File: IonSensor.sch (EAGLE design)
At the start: 20 parts, among them IC1 QUAD_OPAMPD, IC2 QUAD_OPAMPD, IC3 QUAD_OPAMPD, X1 JST-XH-04-PIN-LONG-PAD

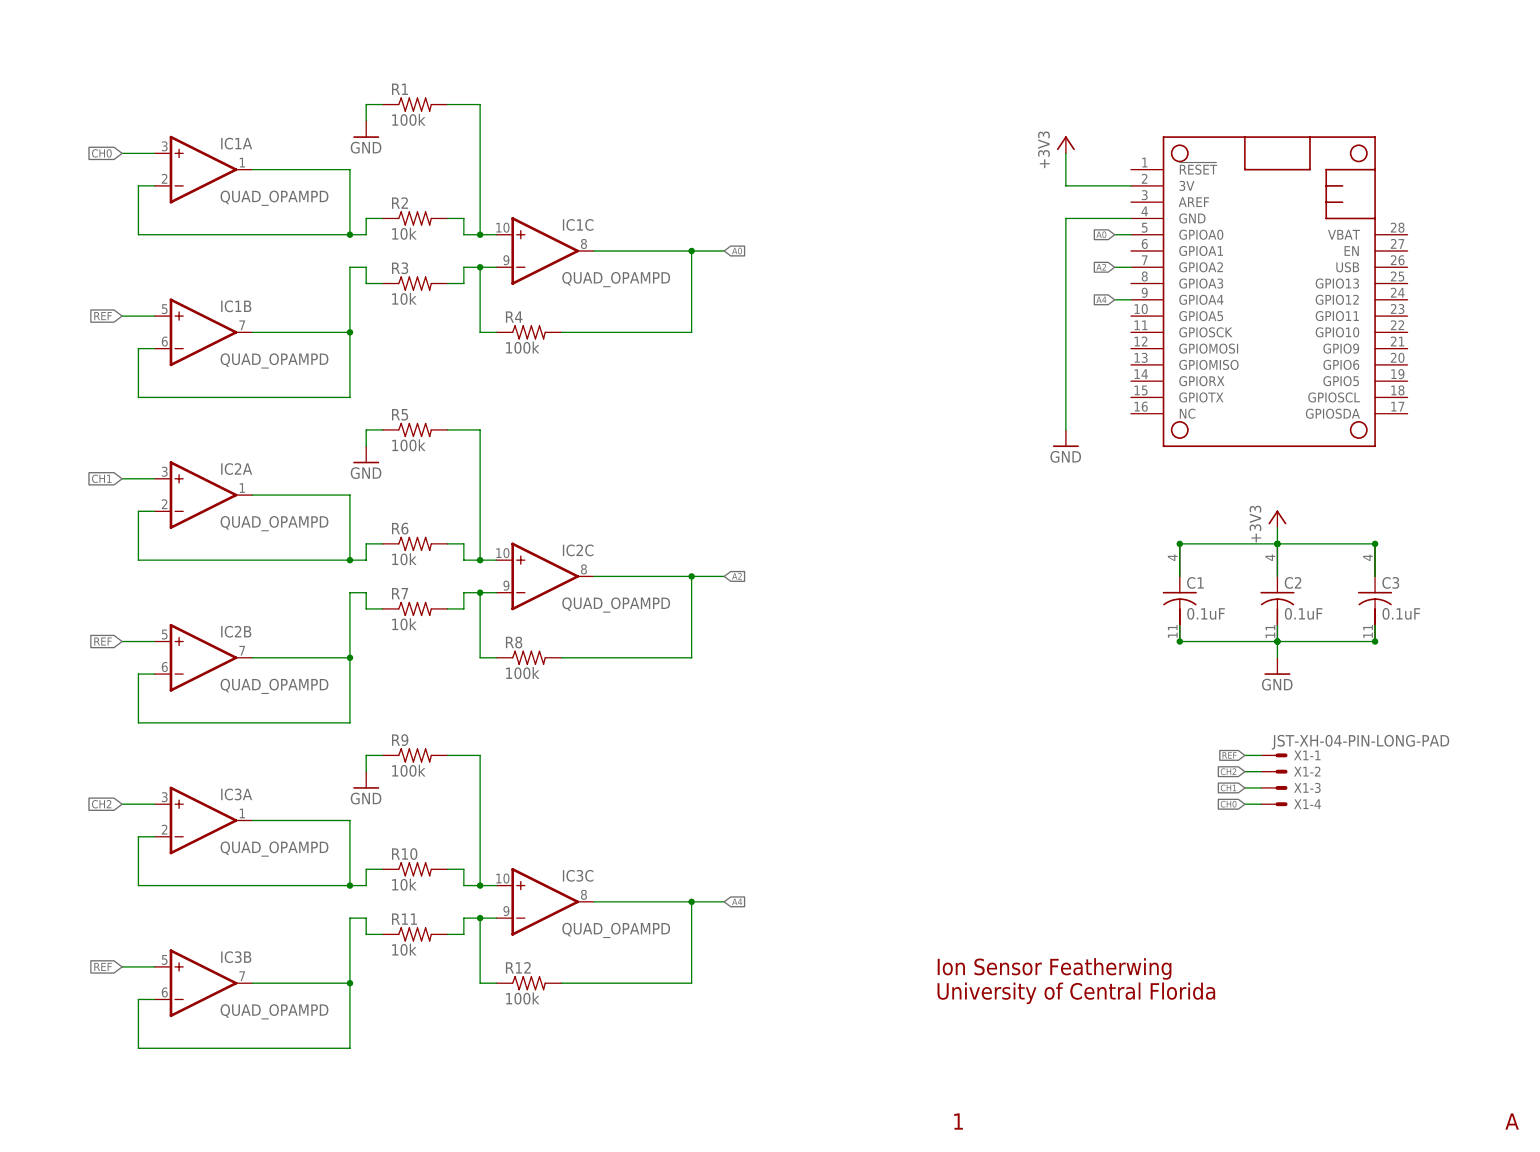
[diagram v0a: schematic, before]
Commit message: Switch to 2 channel opamp
Switched to 2 channel opamp instead of quad opamp.
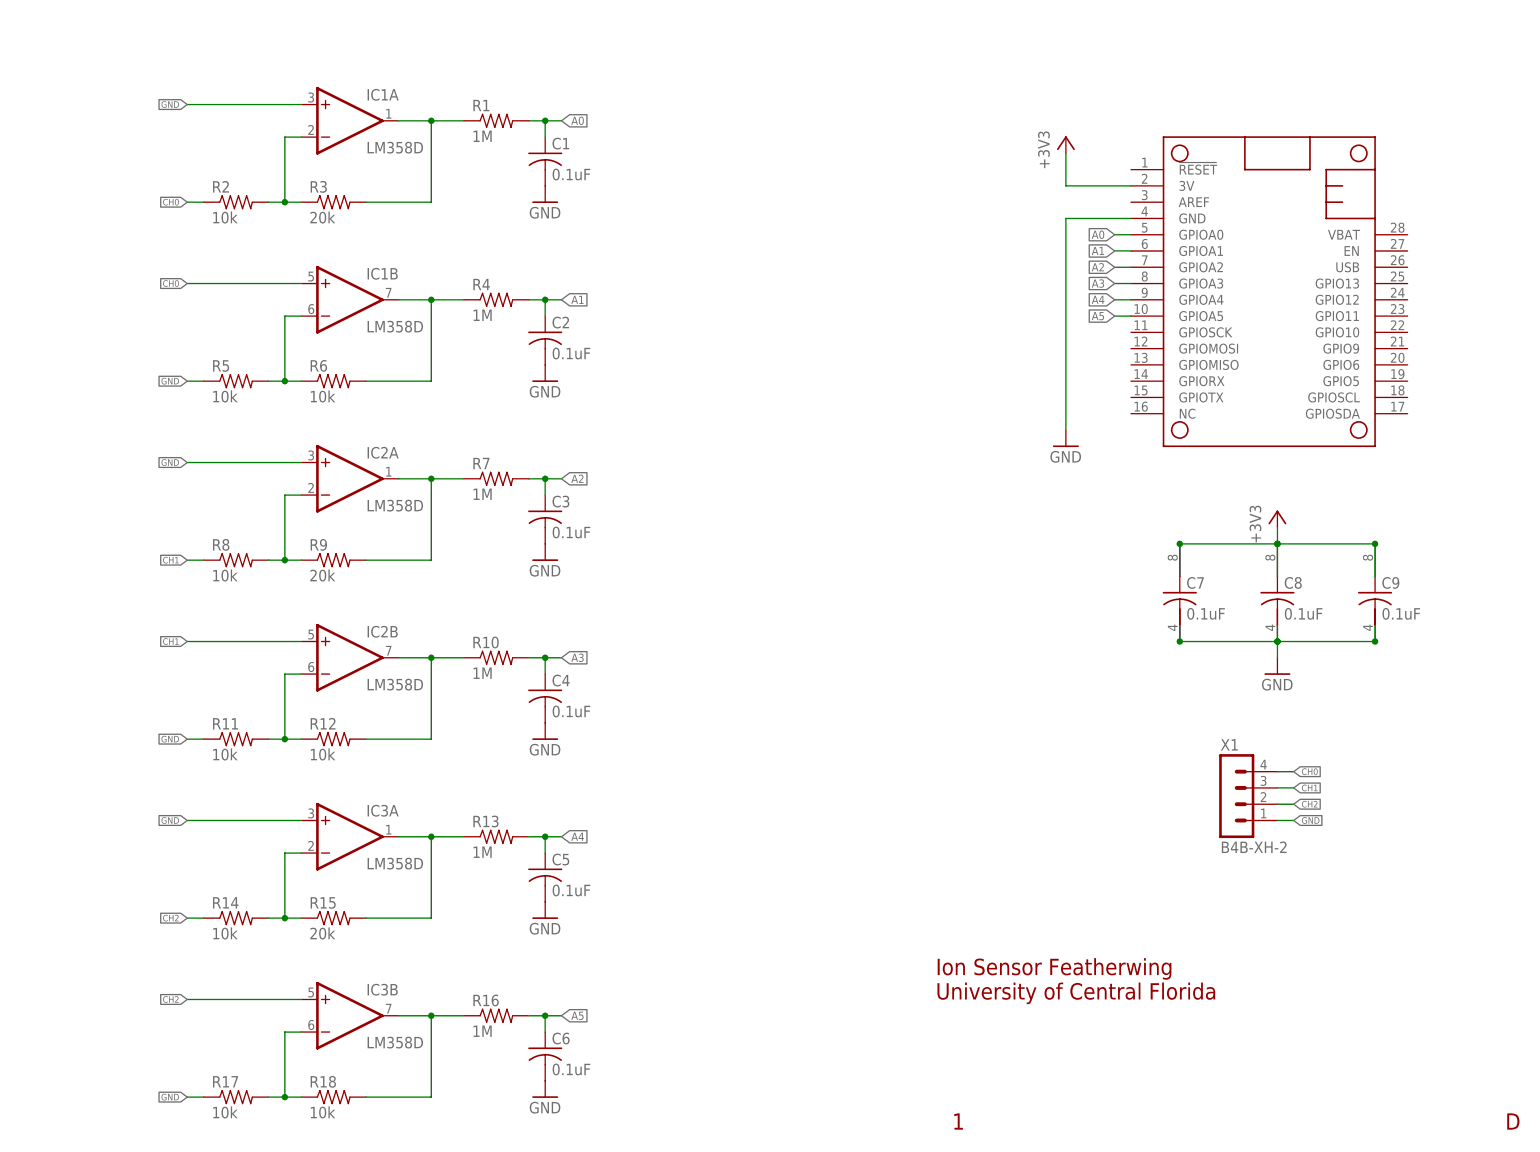
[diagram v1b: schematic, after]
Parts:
- added C4, C5, C6, C7, C8, C9: 0.1uF, adafruit:C-USC0402
- added R13, R16: 1M, adafruit:R-US_R0402
- added R14, R17, R18: 10k, adafruit:R-US_R0402
- added R15: 20k, adafruit:R-US_R0402
- C1, C2, C3: device adafruit:C-USC0603 -> adafruit:C-USC0402
- IC1, IC2, IC3: value QUAD_OPAMPD -> LM358D; device adafruit:QUAD_OPAMPD -> linear:LM358D
- R1, R4: value 100k -> 1M; device adafruit:R-US_R0603 -> adafruit:R-US_R0402
- R10, R7: value 10k -> 1M; device adafruit:R-US_R0603 -> adafruit:R-US_R0402
- R11, R2, R6: device adafruit:R-US_R0603 -> adafruit:R-US_R0402
- R12, R5, R8: value 100k -> 10k; device adafruit:R-US_R0603 -> adafruit:R-US_R0402
- R3: value 10k -> 20k; device adafruit:R-US_R0603 -> adafruit:R-US_R0402
- R9: value 100k -> 20k; device adafruit:R-US_R0603 -> adafruit:R-US_R0402
- X1: value JST-XH-04-PIN-LONG-PAD -> B4B-XH-2; device Rembrandt Electronics - JST XH Connectors v1-0:JST-XH-04-PIN-LONG-PAD -> con-JST XH:B4B-XH-2
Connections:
- removed net N$13: IC3C.+IN, R10.2, R9.2
- removed net N$14: IC3C.-IN, R11.2, R12.1
- removed net REF: IC1B.+IN, IC2B.+IN, IC3B.+IN, X1-1.S
- new net A1: C2.1, MS1.GPIOA1, R4.2
- new net A3: C4.1, MS1.GPIOA3, R10.2
- new net A5: C6.1, MS1.GPIOA5, R16.2
- new net N$10: IC3A.OUT, R13.1, R15.2
- new net N$5: IC2A.-IN, R8.2, R9.1
- net +3V3: now also C7.1, C8.1, C9.1; no longer C1.1, C2.1, C3.1
- net A0: now also C1.1, R1.2; no longer IC1C.OUT, R4.2
- net A2: now also C3.1, R7.2; no longer IC2C.OUT, R8.2
- net A4: now also C5.1, R13.2; no longer IC3C.OUT, R12.2
- net CH0: now also IC1B.+IN, R2.1, X1.4; no longer IC1A.+IN, X1-4.S
- net CH1: now also IC2B.+IN, R8.1, X1.3; no longer IC2A.+IN, X1-3.S
- net CH2: now also IC3B.+IN, R14.1, X1.2; no longer IC3A.+IN, X1-2.S
- net GND: now also C4.2, C5.2, C6.2, C7.2, C8.2, C9.2, IC1A.+IN, IC2A.+IN, IC3A.+IN, R11.1, R17.1, X1.1; no longer R1.1, R9.1
- net N$1: now also R2.2, R3.1; no longer IC1A.OUT, R2.1
- net N$11: now also IC3B.-IN, R17.2, R18.1; no longer IC3A.-IN, IC3A.OUT, R10.1
- net N$12: now also R16.1, R18.2; no longer IC3B.-IN, R11.1
- net N$2: now also IC1B.-IN, R5.2, R6.1; no longer IC1C.+IN, R1.2, R2.2
- net N$3: now also IC1A.OUT, R1.1, R3.2; no longer IC1B.-IN, IC1B.OUT, R3.1
- net N$4: now also IC1B.OUT, R6.2; no longer IC1C.-IN, R3.2
- net N$6: now also R7.1, R9.2; no longer IC2A.-IN, R6.1
- net N$7: now also R11.2, R12.1; no longer IC2B.OUT, R7.1
- net N$8: now also IC2B.OUT, R10.1, R12.2; no longer IC2C.+IN, R5.2, R6.2
- net N$9: now also IC3A.-IN, R14.2, R15.1; no longer IC2C.-IN, R7.2, R8.1
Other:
- note added: "D"
- note removed: "A"
- moved on the sheet: C1, C2, C3, IC1A, IC1B, IC2A, IC2B, IC3A, IC3B, R1, R10, R11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

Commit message: Revert "Switch to 2 channel opamp"
This reverts commit d2c6276b5e9005aaa4bb267ec01d57cf95291150.
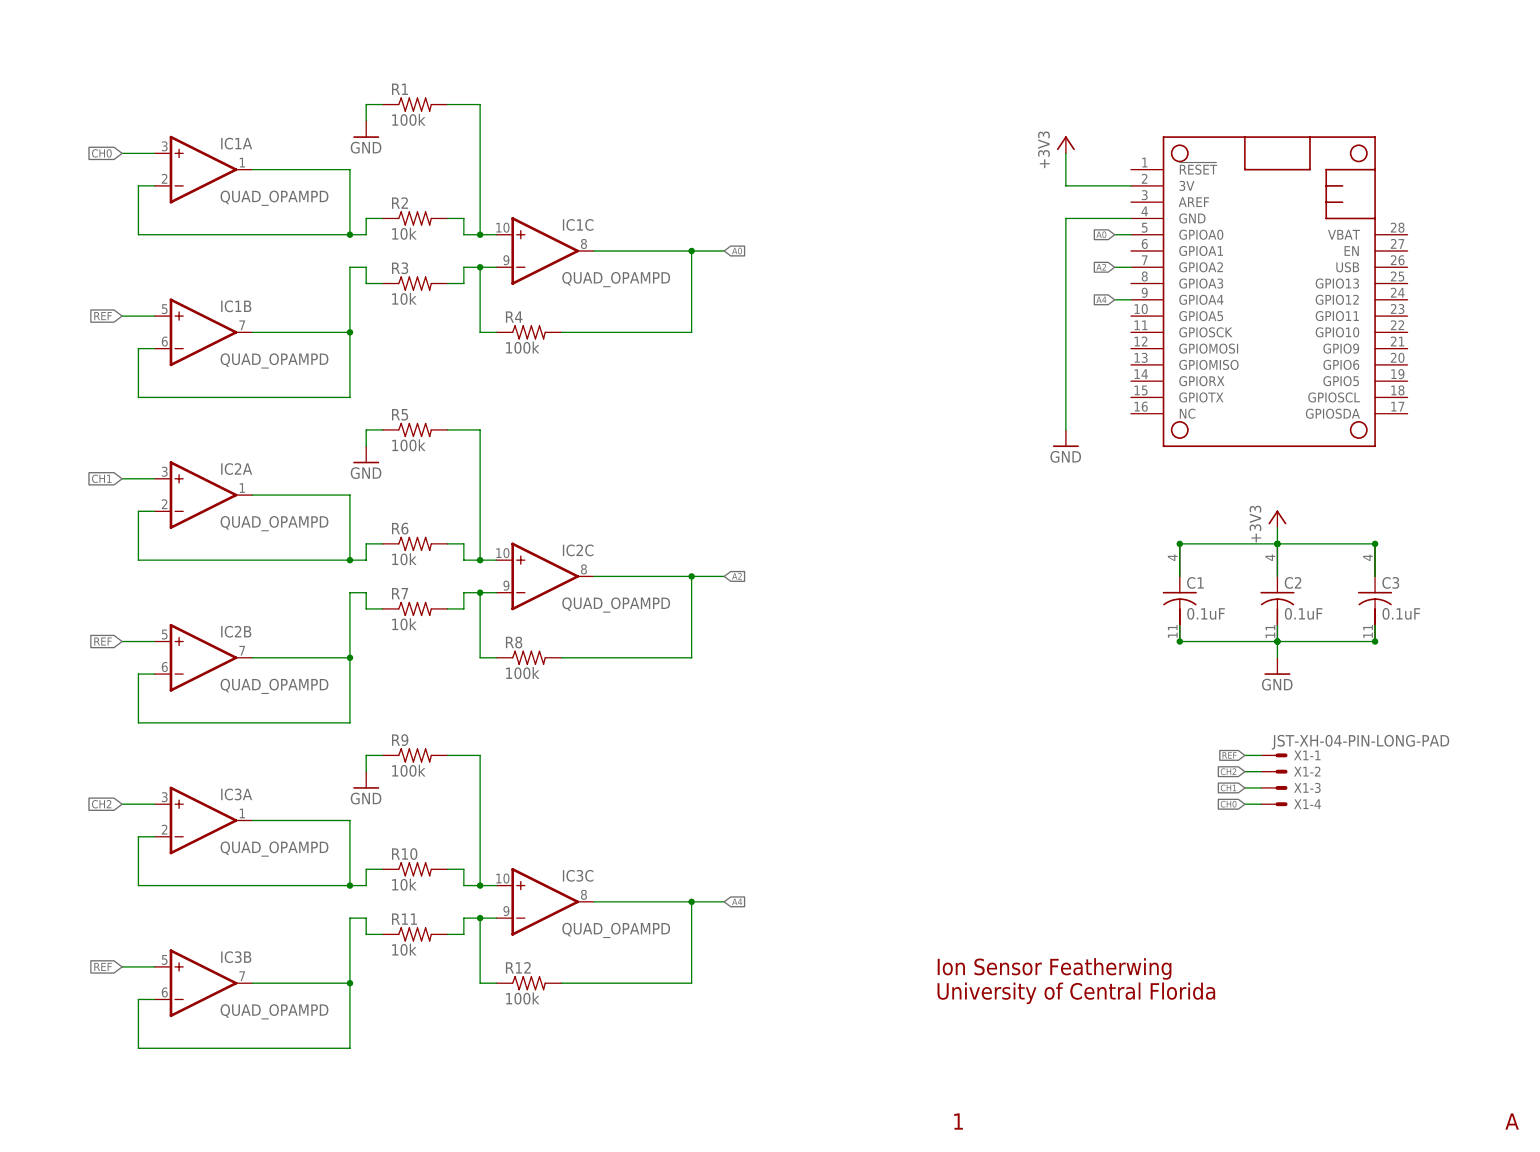
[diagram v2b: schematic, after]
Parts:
- removed C4, C5, C6, C7, C8, C9: 0.1uF, adafruit:C-USC0402
- removed R13, R16: 1M, adafruit:R-US_R0402
- removed R14, R17, R18: 10k, adafruit:R-US_R0402
- removed R15: 20k, adafruit:R-US_R0402
- C1, C2, C3: device adafruit:C-USC0402 -> adafruit:C-USC0603
- IC1, IC2, IC3: value LM358D -> QUAD_OPAMPD; device linear:LM358D -> adafruit:QUAD_OPAMPD
- R1, R4: value 1M -> 100k; device adafruit:R-US_R0402 -> adafruit:R-US_R0603
- R10, R7: value 1M -> 10k; device adafruit:R-US_R0402 -> adafruit:R-US_R0603
- R11, R2, R6: device adafruit:R-US_R0402 -> adafruit:R-US_R0603
- R12, R5, R8: value 10k -> 100k; device adafruit:R-US_R0402 -> adafruit:R-US_R0603
- R3: value 20k -> 10k; device adafruit:R-US_R0402 -> adafruit:R-US_R0603
- R9: value 20k -> 100k; device adafruit:R-US_R0402 -> adafruit:R-US_R0603
- X1: value B4B-XH-2 -> JST-XH-04-PIN-LONG-PAD; device con-JST XH:B4B-XH-2 -> Rembrandt Electronics - JST XH Connectors v1-0:JST-XH-04-PIN-LONG-PAD
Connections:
- removed net A1: C2.1, MS1.GPIOA1, R4.2
- removed net A3: C4.1, MS1.GPIOA3, R10.2
- removed net A5: C6.1, MS1.GPIOA5, R16.2
- removed net N$10: IC3A.OUT, R13.1, R15.2
- removed net N$5: IC2A.-IN, R8.2, R9.1
- new net N$13: IC3C.+IN, R10.2, R9.2
- new net N$14: IC3C.-IN, R11.2, R12.1
- new net REF: IC1B.+IN, IC2B.+IN, IC3B.+IN, X1-1.S
- net +3V3: now also C1.1, C2.1, C3.1; no longer C7.1, C8.1, C9.1
- net A0: now also IC1C.OUT, R4.2; no longer C1.1, R1.2
- net A2: now also IC2C.OUT, R8.2; no longer C3.1, R7.2
- net A4: now also IC3C.OUT, R12.2; no longer C5.1, R13.2
- net CH0: now also IC1A.+IN, X1-4.S; no longer IC1B.+IN, R2.1, X1.4
- net CH1: now also IC2A.+IN, X1-3.S; no longer IC2B.+IN, R8.1, X1.3
- net CH2: now also IC3A.+IN, X1-2.S; no longer IC3B.+IN, R14.1, X1.2
- net GND: now also R1.1, R9.1; no longer C4.2, C5.2, C6.2, C7.2, C8.2, C9.2, IC1A.+IN, IC2A.+IN, IC3A.+IN, R11.1, R17.1, X1.1
- net N$1: now also IC1A.OUT, R2.1; no longer R2.2, R3.1
- net N$11: now also IC3A.-IN, IC3A.OUT, R10.1; no longer IC3B.-IN, R17.2, R18.1
- net N$12: now also IC3B.-IN, R11.1; no longer R16.1, R18.2
- net N$2: now also IC1C.+IN, R1.2, R2.2; no longer IC1B.-IN, R5.2, R6.1
- net N$3: now also IC1B.-IN, IC1B.OUT, R3.1; no longer IC1A.OUT, R1.1, R3.2
- net N$4: now also IC1C.-IN, R3.2; no longer IC1B.OUT, R6.2
- net N$6: now also IC2A.-IN, R6.1; no longer R7.1, R9.2
- net N$7: now also IC2B.OUT, R7.1; no longer R11.2, R12.1
- net N$8: now also IC2C.+IN, R5.2, R6.2; no longer IC2B.OUT, R10.1, R12.2
- net N$9: now also IC2C.-IN, R7.2, R8.1; no longer IC3A.-IN, R14.2, R15.1
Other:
- note added: "A"
- note removed: "D"
- moved on the sheet: C1, C2, C3, IC1A, IC1B, IC2A, IC2B, IC3A, IC3B, R1, R10, R11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
